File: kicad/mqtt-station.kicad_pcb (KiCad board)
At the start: 2 copper layers, 65 x 56 mm, 21 parts, among them J101 Conn_01x04, J102 Conn_02x07_Odd_Even, J103 Conn_01x02, J104 Conn_01x06, P1 Conn_02x20_Odd_Even, Q101 Q_NMOS_GSD, Q102 Q_PMOS_GSD, Q103 Q_PMOS_GSD, Q104 Q_PMOS_GSD, U101 ESP-WROOM-32

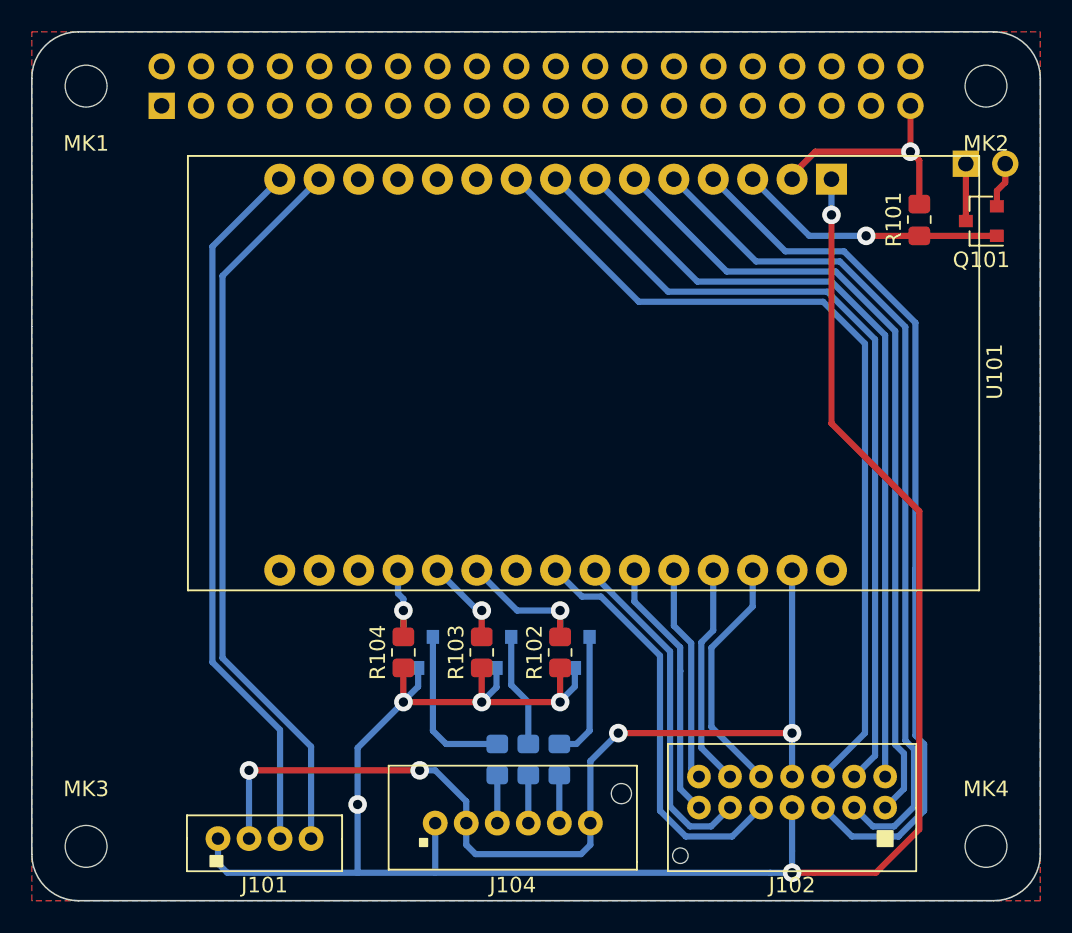
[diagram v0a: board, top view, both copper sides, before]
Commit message: wip
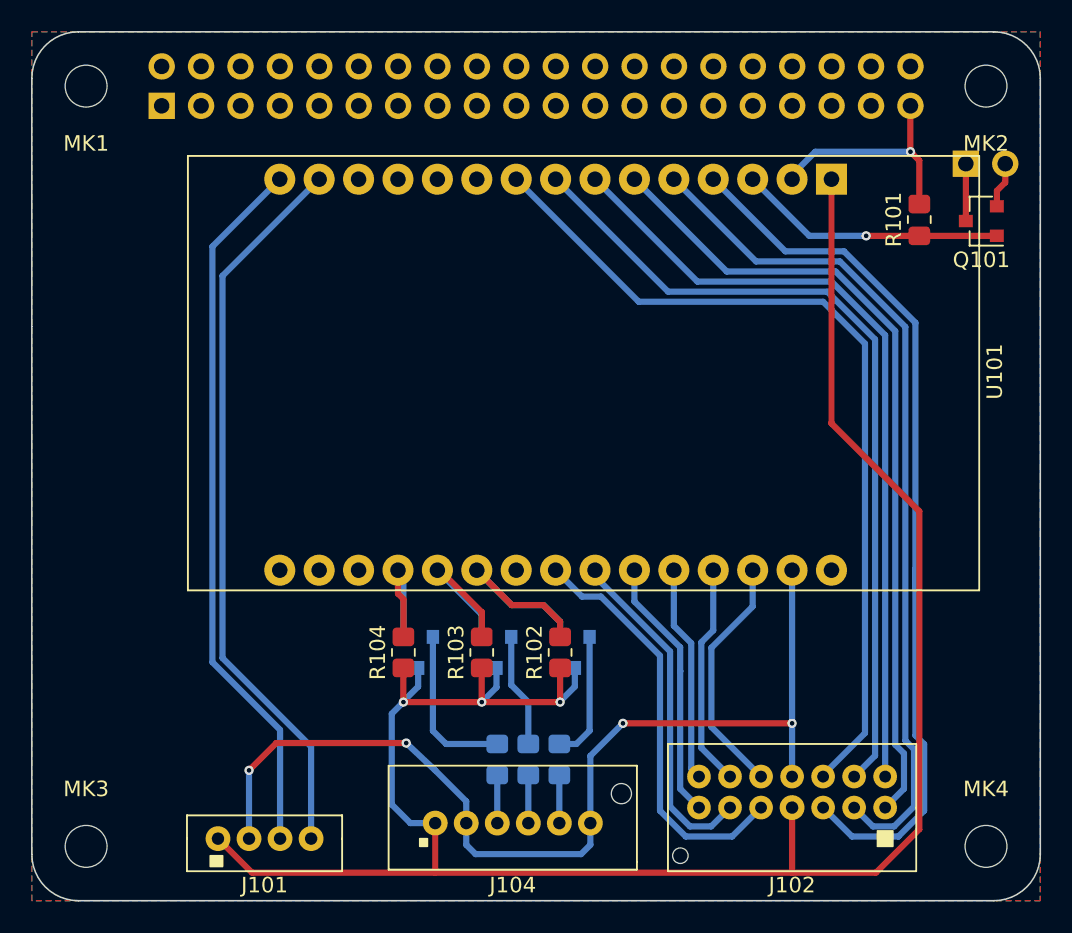
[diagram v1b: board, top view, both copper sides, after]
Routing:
- net GND: track 86.4 -> 80.0 mm
- net /pwm_led_re: track 9.85 -> 15.5 mm, vias 1 -> 0
- net /pwm_led_bl: track 7.34 -> 11.1 mm, vias 1 -> 0
- net +3V3: track 136.6 -> 133.6 mm, vias 6 -> 3
- net /pwm_led_gr: track 6.14 -> 8.89 mm, vias 1 -> 0
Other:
- net class Default: via_dia 1.2 -> 0.6; via_drill 0.6 -> 0.3
